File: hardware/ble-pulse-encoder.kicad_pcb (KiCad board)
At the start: 2 copper layers, 39 x 39 mm, 59 parts, among them J1 USB_B_Micro, J2 EZmate-3, J3 EZmate-4, J4 TC2030-IDC-NL, J5 EZmate-5, Q1 BSS84, Q2 Q_Photo_NPN_CBE, Q3 Q_Photo_NPN_CBE, SW1 SW_Push, SW2 SW_Push, U1 STBC08, U2 nRF52832-QFxx, U3 MIC5301, Y1 32.768kHz, Y2 32MHz

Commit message: hw: assembly notes
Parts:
- D6: value Green -> Yellow
- R10, R9: value 1k -> 470
- R11, R12: value 1k -> 10k
- U3: value MIC5301 -> TPS7A0333DBVR
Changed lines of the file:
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@@
         (effects (font (size 1 1) (thickness 0.15)))
     )
-    (fp_text value "1k" (at 0 1.43) (layer "F.Fab")
+    (fp_text value "10k" (at 0 1.43) (layer "F.Fab")
         (effects (font (size 1 1) (thickness 0.15)))
     )
@@
         (effects (font (size 1 1) (thickness 0.15)))
     )
-    (fp_text value "1k" (at 0 1.43 90) (layer "F.Fab")
+    (fp_text value "470" (at 0 1.43 90) (layer "F.Fab")
         (effects (font (size 1 1) (thickness 0.15)))
     )
@@
         (effects (font (size 1 1) (thickness 0.15)))
     )
-    (fp_text value "MIC5301" (at 0 2.4 90) (layer "F.Fab")
+    (fp_text value "TPS7A0333DBVR" (at 0 2.4 90) (layer "F.Fab")
         (effects (font (size 1 1) (thickness 0.15)))
     )
@@
         (effects (font (size 1 1) (thickness 0.15)))
     )
-    (fp_text value "Green" (at 0 1.43 90) (layer "F.Fab")
+    (fp_text value "Yellow" (at 0 1.43 90) (layer "F.Fab")
         (effects (font (size 1 1) (thickness 0.15)))
     )
@@
         (effects (font (size 1 1) (thickness 0.15)))
     )
-    (fp_text value "1k" (at 0 1.43 90) (layer "F.Fab")
+    (fp_text value "470" (at 0 1.43 90) (layer "F.Fab")
         (effects (font (size 1 1) (thickness 0.15)))
     )
@@
         (effects (font (size 1 1) (thickness 0.15)))
     )
-    (fp_text value "1k" (at 0 1.43) (layer "F.Fab")
-        (effects (font (size 1 1) (thickness 0.15)))
-    )
+    (fp_text value "10k" (at 0 1.43) (layer "F.Fab")
+        (effects (font (size 1 1) (thickness 0.15)))
+    )

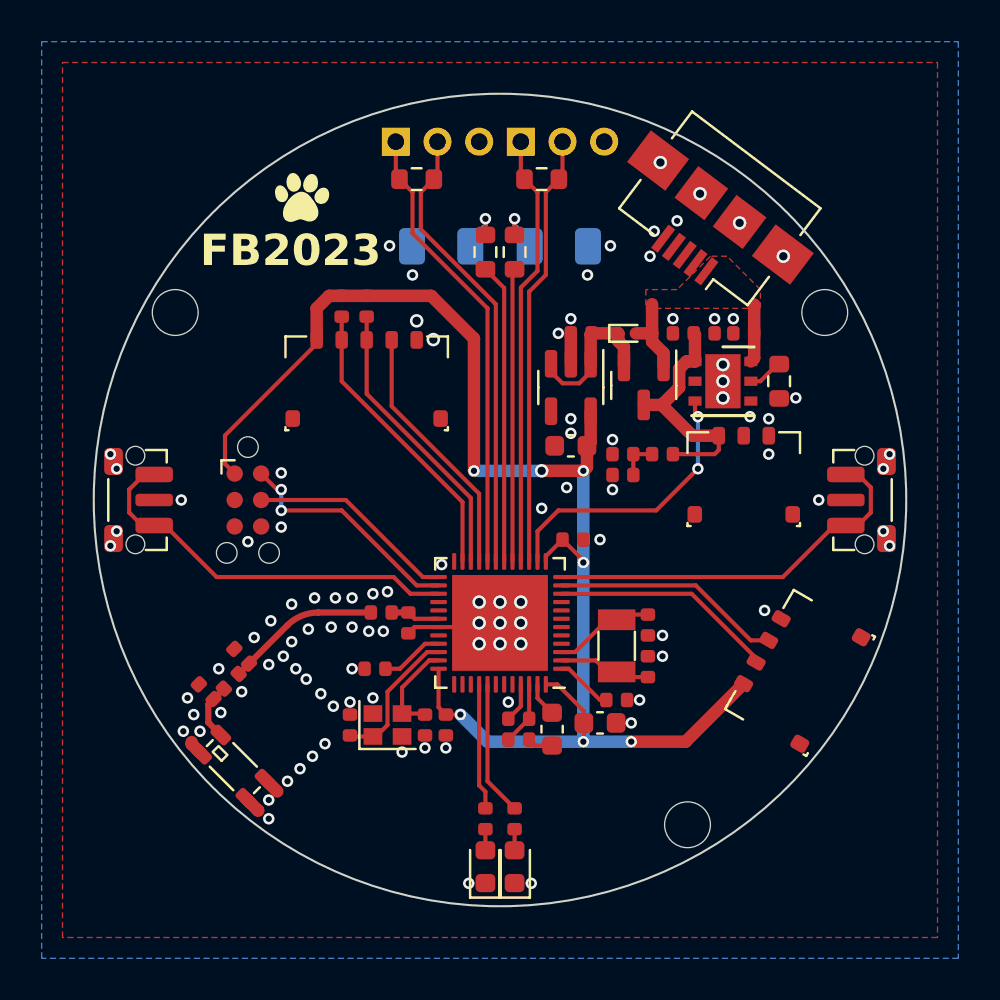
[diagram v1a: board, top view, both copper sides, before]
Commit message: hw: r1
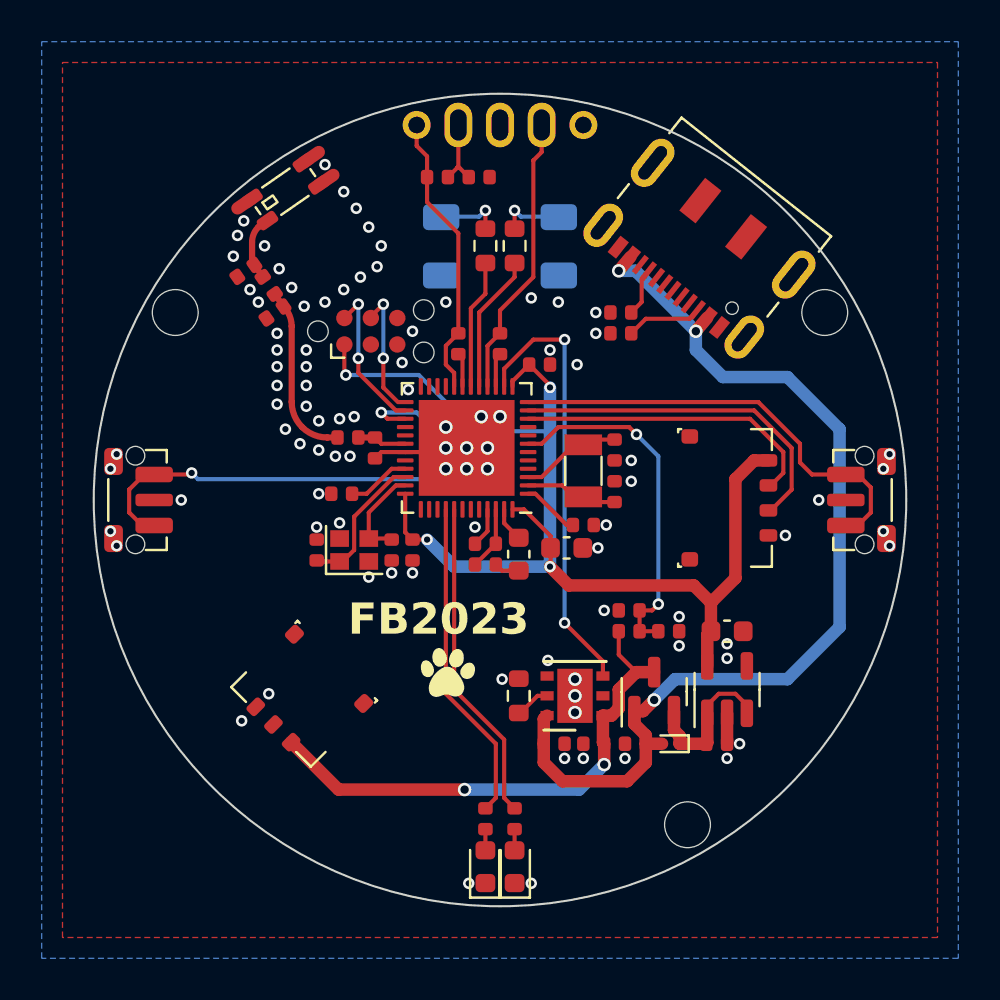
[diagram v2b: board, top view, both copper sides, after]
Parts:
- removed J5: EZmate-5, balto:EZmate-5
- removed Q2, Q3: Q_Photo_NPN_CBE, Connector_PinHeader_2.00mm:PinHeader_1x03_P2.00mm_Vertical
- removed R7, R8: 4.7k, balto:R_0402_Worthington
- added J6: USB_C_Receptacle_USB2.0, Connector_USB:USB_C_Receptacle_JAE_DX07S016JA1R1500, F.Cu at (159.0, 78.4)
- added R14: 5.1k, balto:R_0402_Worthington, F.Cu at (154.8, 83.0)
- added R15: 0, balto:R_0402_Worthington, F.Cu at (146.0, 75.5)
- added R16: 0, balto:R_0402_Worthington, F.Cu at (148.0, 75.5)
- added R2: 5.1k, balto:R_0402_Worthington, F.Cu at (154.8, 82.0)
- AE1: footprint balto:2450AT18D0100001-R -> balto:2450AT18D0100001-L
- J1: value USB_B_Micro -> Conn_01x05; footprint Connector_USB:USB_Micro-B_Amphenol_10104110_Horizontal -> Connector_PinHeader_2.00mm:PinHeader_1x05_P2.00mm_Vertical; moved to B.Cu
- R11, R12: footprint Resistor_SMD:R_0603_1608Metric -> balto:R_0402_Worthington
- moved AE1 27.7 mm to (138.7, 76.2), turned to 34.8 degrees
- moved G*** 23.9 mm to (146.5, 99.3)
- moved J2 23.5 mm to (139.6, 100.3), turned to 135 degrees
- moved C6 21.7 mm to (151.6, 102.7), turned to 0 degrees
- moved C17 20.7 mm to (159.4, 102.7), turned to 0 degrees
- moved C12 20.4 mm to (153.5, 102.7), turned to 180 degrees
- moved C16 20.3 mm to (136.8, 80.0), turned to -145 degrees
- moved D3 19.8 mm to (157.2, 102.7), turned to 180 degrees
- moved R5 19.7 mm to (155.5, 102.7), turned to 180 degrees
- moved R1 19.6 mm to (149.9, 100.4), turned to 90 degrees
- moved L4 19.1 mm to (137.9, 80.7), turned to -55 degrees
- moved U1 16.7 mm to (152.6, 100.4), turned to 180 degrees
- moved C14 16.6 mm to (138.2, 82.0), turned to -145 degrees
- moved U3 16.3 mm to (159.9, 100.1), turned to 90 degrees
- moved Q1 14.7 mm to (156.4, 100.2), turned to 90 degrees
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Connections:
- J1 pad 1: +5V -> /PH1_SENSE
- J1 pad 2: unconnected-(J1-D--Pad2) -> Net-(J1-Pin_2)
- J1 pad 3: unconnected-(J1-D+-Pad3) -> GND
- J1 pad 4: unconnected-(J1-ID-Pad4) -> /PH0_SENSE
- U2 pad 21: /EXT_IRQ -> unconnected-(U2-P0.18/SWO-Pad21)
- U2 pad 22: /SDA -> unconnected-(U2-P0.19-Pad22)
- U2 pad 23: /SCL -> unconnected-(U2-P0.20-Pad23)
- U2 pad 7: unconnected-(U2-P0.05/AIN3-Pad7) -> /ADC_VBATT
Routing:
- net +5V: track 6.77 -> 48.5 mm, vias 0 -> 3
- net /PH1_PWR: track 22.0 -> 1.63 mm
- net /PH0_PWR: track 20.8 -> 1.63 mm
- net /ADC_VBATT: track 1.90 -> 17.2 mm, vias 0 -> 2
- net /SCL: track 14.2 -> 0.00 mm
- net +3V3: track 71.3 -> 57.2 mm, vias 7 -> 4
- net /SDA: track 13.8 -> 0.00 mm
- net +BATT: track 11.5 -> 25.0 mm, vias 0 -> 2
- net /EXT_IRQ: track 12.4 -> 0.00 mm
- net /LED_A: track 6.07 -> 15.6 mm
- net /LED_B: track 6.49 -> 15.6 mm
- net /D1_PWR: track 14.4 -> 6.21 mm
- net /PH1_SENSE: track 22.0 -> 13.8 mm
- net /CHRG: track 13.7 -> 21.2 mm
- net /D0_PWR: track 14.1 -> 6.63 mm
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- removed copper zone on F.Cu, net +5V
